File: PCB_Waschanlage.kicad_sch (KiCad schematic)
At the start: 81 parts, among them J10 JMPR_LED_BTN_Sensor_1, J11 JMPR_LED_BTN_Sensor_4, J12 Conn_LED_Error, J13 Conn_LED_MainWash, J14 Conn_BTN_Start, J15 Conn_BTN_Basic, J16 Conn_LED_Motor, J17 Conn_LED_Red, J18 Conn_BTN_Sensor_1, J19 Conn_BTN_Sensor_4, J20 JMPR_LED_PreWash, J21 JMPR_LED_Start, J22 JMPR_LED_Basic, J23 JMPR_LED_BTN_On_Off, J24 JMPR_LED_BTN_Special, J25 JMPR_LED_Green, J26 JMPR_LED_BTN_Sensor_2, J27 JMPR_LED_BTN_Sensor_5, J28 Conn_LED_PreWash, J29 Conn_LED_Start, J3 Conn_Fuse, J30 Conn_LED_Basic, J31 Conn_BTN_On_Off, J32 Conn_BTN_Special, J33 Conn_LED_Green, J34 Conn_BTN_Sensor_2, J35 Conn_BTN_Sensor_5, J36 JMPR_LED_Special, J37 JMPR_LED_Care, J38 JMPR_LED_Underbody, J39 JMPR_LED_BTN_EmergencyOff, J4 JMPR_LED_Error, J40 JMPR_LED_BTN_Premium, J41 JMPR_LED_BTN_Sensor_3, J42 Conn_LED_Special, J43 Conn_LED_Care, J44 Conn_LED_Underbody, J45 Conn_BTN_EmergencyOff, J46 Conn_BTN_Premium, J47 Conn_BTN_Sensor_3, J48 JMPR_LED_Rims, J49 JMPR_LED_Premium, J5 JMPR_LED_MainWash, J50 JMPR_LED_Dry, J51 Conn_LED_Rims, J52 Conn_LED_Premium, J53 Conn_LED_Dry, J54 Conn_AdditionalPins_1, J55 Conn_AdditionalPins_2, J56 Conn_AdditionalPins_3, J57 5103308-6, J58 5103308-6, J6 JMPR_LED_BTN_Start, J7 JMPR_LED_BTN_Basic, J8 JMPR_LED_Motor, J9 JMPR_LED_Red

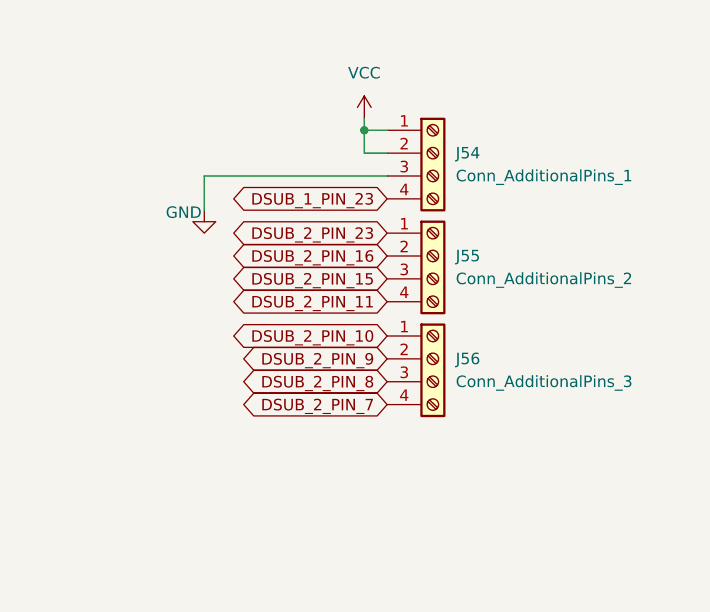
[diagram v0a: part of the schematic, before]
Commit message: Routing fimished
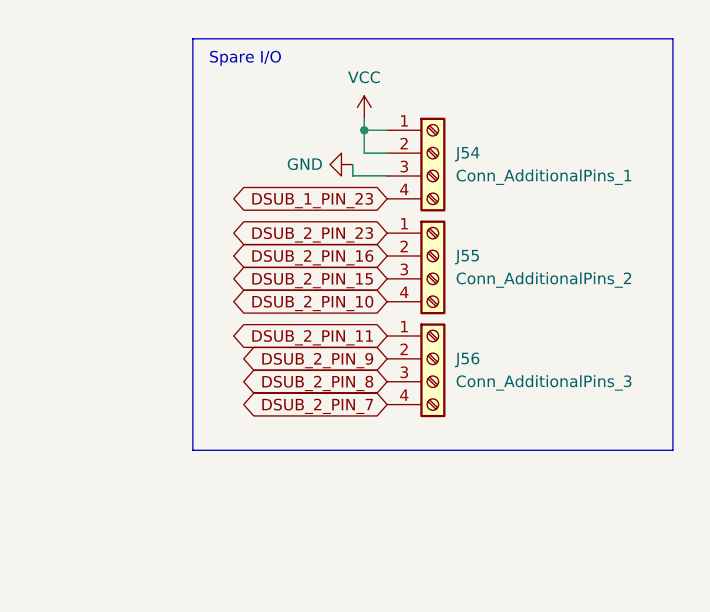
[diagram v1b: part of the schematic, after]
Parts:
- J54, J55, J56: footprint TerminalBlock:TerminalBlock_MaiXu_MX126-5.0-04P_1x04_P5.00mm -> TBL002A-350-04GY-2GY:CUI_TBL002A-350-04GY-2GY
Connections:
- net DSUB_2_PIN_10: now also J55.4 (Pin_4); no longer J56.1 (Pin_1)
- net DSUB_2_PIN_11: now also J56.1 (Pin_1); no longer J55.4 (Pin_4)
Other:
- note added: "Spare I/O"
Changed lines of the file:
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@@
 	(generator_version "10.0")
 	(paper "A3")
+	(rectangle
+		(start 318.77 22.86)
+		(end 372.11 68.58)
+		(stroke
+			(width 0)
+			(type default)
+		)
+		(fill
+			(type none)
+		)
+	)
+	(text "Spare I/O"
+		(exclude_from_sim no)
+		(at 324.612 25.146 0)
+		(effects
+			(font
+				(size 1.27 1.27)
+			)
+		)
+	)
 	(junction
 		(at 208.28 116.84)
@@
 	(wire
 		(pts
-			(xy 320.04 41.91) (xy 320.04 38.1)
+			(xy 336.55 36.83) (xy 336.55 38.1)
 		)
 		(stroke
@@
 	(wire
 		(pts
-			(xy 320.04 38.1) (xy 340.36 38.1)
+			(xy 336.55 38.1) (xy 340.36 38.1)
 		)
 		(stroke
@@
 		)
 	)
+	(global_label "DSUB_2_PIN_11"
+		(shape bidirectional)
+		(at 340.36 55.88 180)
+		(fields_autoplaced yes)
+		(effects
+			(font
+				(size 1.27 1.27)
+			)
+			(justify right)
+		)
+		(property "Intersheetrefs" "${INTERSHEET_REFS}"
+			(at 321.4469 55.88 0)
+			(hide yes)
+			(show_name no)
+			(do_not_autoplace no)
+			(effects
+				(font
+					(size 1.27 1.27)
+				)
+				(justify right)
+			)
+		)
+	)
 	(global_label "DSUB_2_PIN_8"
 		(shape bidirectional)
@@
 		)
 	)
-	(global_label "DSUB_2_PIN_10"
-		(shape bidirectional)
-		(at 340.36 55.88 180)
-		(fields_autoplaced yes)
-		(effects
-			(font
-				(size 1.27 1.27)
-			)
-			(justify right)
-		)
-		(property "Intersheetrefs" "${INTERSHEET_REFS}"
-			(at 321.4469 55.88 0)
-			(hide yes)
-			(show_name no)
-			(do_not_autoplace no)
-			(effects
-				(font
-					(size 1.27 1.27)
-				)
-				(justify right)
-			)
-		)
-	)
 	(global_label "DSUB_2_PIN_16"
 		(shape bidirectional)
@@
 		)
 	)
-	(global_label "LED_Basic"
+	(global_label "DSUB_2_PIN_10"
 		(shape bidirectional)
-		(at 40.64 102.87 180)
+		(at 340.36 52.07 180)
 		(fields_autoplaced yes)
 		(effects
@@
 		)
 		(property "Intersheetrefs" "${INTERSHEET_REFS}"
-			(at 26.9883 102.87 0)
+			(at 321.4469 52.07 0)
 			(hide yes)
 			(show_name no)
@@
 		)
 	)
-	(global_label "BTN_Basic"
+	(global_label "LED_Basic"
 		(shape bidirectional)
-		(at 40.64 190.5 180)
+		(at 40.64 102.87 180)
 		(fields_autoplaced yes)
 		(effects
@@
 		)
 		(property "Intersheetrefs" "${INTERSHEET_REFS}"
-			(at 26.8673 190.5 0)
+			(at 26.9883 102.87 0)
 			(hide yes)
 			(show_name no)
@@
 		)
 	)
-	(global_label "LED_Basic"
+	(global_label "BTN_Basic"
 		(shape bidirectional)
-		(at 172.72 22.86 180)
+		(at 40.64 190.5 180)
 		(fields_autoplaced yes)
 		(effects
@@
 		)
 		(property "Intersheetrefs" "${INTERSHEET_REFS}"
-			(at 159.0683 22.86 0)
+			(at 26.8673 190.5 0)
 			(hide yes)
 			(show_name no)
@@
 		)
 	)
-	(global_label "DSUB_2_PIN_7"
+	(global_label "LED_Basic"
 		(shape bidirectional)
-		(at 340.36 63.5 180)
+		(at 172.72 22.86 180)
 		(fields_autoplaced yes)
 		(effects
@@
 		)
 		(property "Intersheetrefs" "${INTERSHEET_REFS}"
-			(at 322.6564 63.5 0)
+			(at 159.0683 22.86 0)
 			(hide yes)
 			(show_name no)
@@
 		)
 	)
-	(global_label "LED_Care"
+	(global_label "DSUB_2_PIN_7"
 		(shape bidirectional)
-		(at 214.63 43.18 180)
+		(at 340.36 63.5 180)
 		(fields_autoplaced yes)
 		(effects
@@
 		)
 		(property "Intersheetrefs" "${INTERSHEET_REFS}"
-			(at 201.825 43.18 0)
+			(at 322.6564 63.5 0)
 			(hide yes)
 			(show_name no)
@@
 		)
 	)
-	(global_label "DSUB_2_PIN_11"
+	(global_label "LED_Care"
 		(shape bidirectional)
-		(at 340.36 52.07 180)
+		(at 214.63 43.18 180)
 		(fields_autoplaced yes)
 		(effects
@@
 		)
 		(property "Intersheetrefs" "${INTERSHEET_REFS}"
-			(at 321.4469 52.07 0)
+			(at 201.825 43.18 0)
 			(hide yes)
 			(show_name no)
@@
 			)
 		)
-		(property "Footprint" "TerminalBlock:TerminalBlock_MaiXu_MX126-5.0-04P_1x04_P5.00mm"
+		(property "Footprint" "TBL002A-350-04GY-2GY:CUI_TBL002A-350-04GY-2GY"
 			(at 345.44 35.56 0)
 			(hide yes)
@@
 			)
 		)
-		(property "Footprint" "TerminalBlock:TerminalBlock_MaiXu_MX126-5.0-04P_1x04_P5.00mm"
+		(property "Footprint" "TBL002A-350-04GY-2GY:CUI_TBL002A-350-04GY-2GY"
 			(at 345.44 58.42 0)
 			(hide yes)
@@
 			)
 		)
-		(property "Footprint" "TerminalBlock:TerminalBlock_MaiXu_MX126-5.0-04P_1x04_P5.00mm"
+		(property "Footprint" "TBL002A-350-04GY-2GY:CUI_TBL002A-350-04GY-2GY"
 			(at 345.44 46.99 0)
 			(hide yes)
@@
 	(symbol
 		(lib_id "power:GND")
-		(at 320.04 41.91 0)
+		(at 336.55 36.83 270)
 		(unit 1)
 		(body_style 1)
@@
 		(dnp no)
 		(property "Reference" "#PWR037"
-			(at 320.04 48.26 0)
+			(at 330.2 36.83 0)
 			(hide yes)
 			(show_name no)
@@
 		)
 		(property "Value" "GND"
-			(at 317.754 42.164 0)
+			(at 331.216 36.83 90)
 			(show_name no)
 			(do_not_autoplace no)
@@
 		)
 		(property "Footprint" ""
-			(at 320.04 41.91 0)
+			(at 336.55 36.83 0)
 			(hide yes)
 			(show_name no)
@@
 		)
 		(property "Datasheet" ""
-			(at 320.04 41.91 0)
+			(at 336.55 36.83 0)
 			(hide yes)
 			(show_name no)
@@
 		)
 		(property "Description" "Power symbol creates a global label with name \"GND\" , ground"
-			(at 320.04 41.91 0)
+			(at 336.55 36.83 0)
 			(hide yes)
 			(show_name no)
@@
 		(in_pos_files yes)
 		(dnp no)
-		(fields_autoplaced yes)
 		(property "Reference" "#PWR038"
 			(at 337.82 35.56 0)
@@
 		)
 		(property "Value" "VCC"
-			(at 337.82 26.67 0)
+			(at 337.82 27.178 0)
 			(show_name no)
 			(do_not_autoplace no)
